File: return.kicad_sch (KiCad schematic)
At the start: 46 parts, among them IC1 LC709203F/MH, Q3 MOSFET-P, SW1 SWITCH_TACT_SMT4.6X2.8, SW2 SWITCH_TACT_SMT4.6X2.8, SW3 SW_Push, U1 ESP32-S3-MINI-1, U2 VREG_SOT23-5, U3 MCP73831/2, U4 BME280, U5 VREG_SOT23-5, X1 JSTPH, X3 USB_C

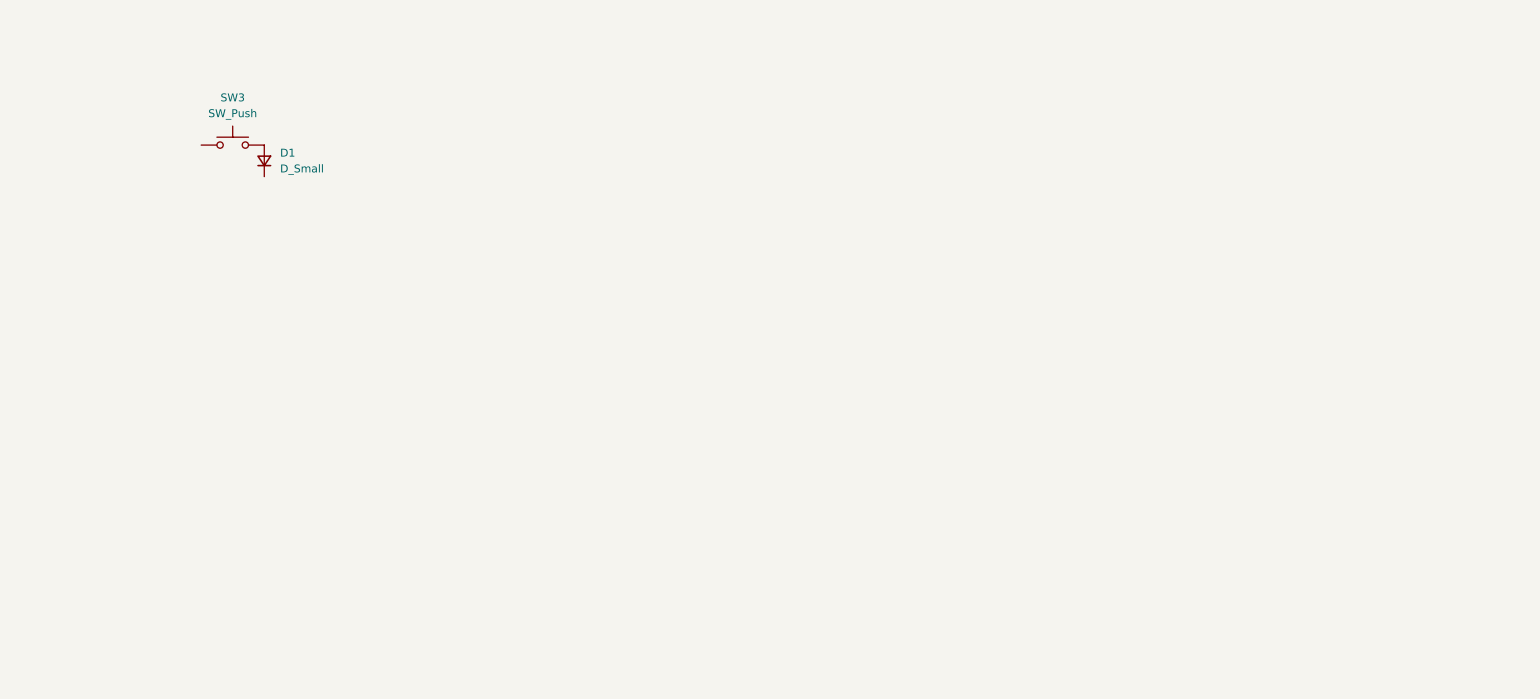
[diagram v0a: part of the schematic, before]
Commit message: Revise Schematic
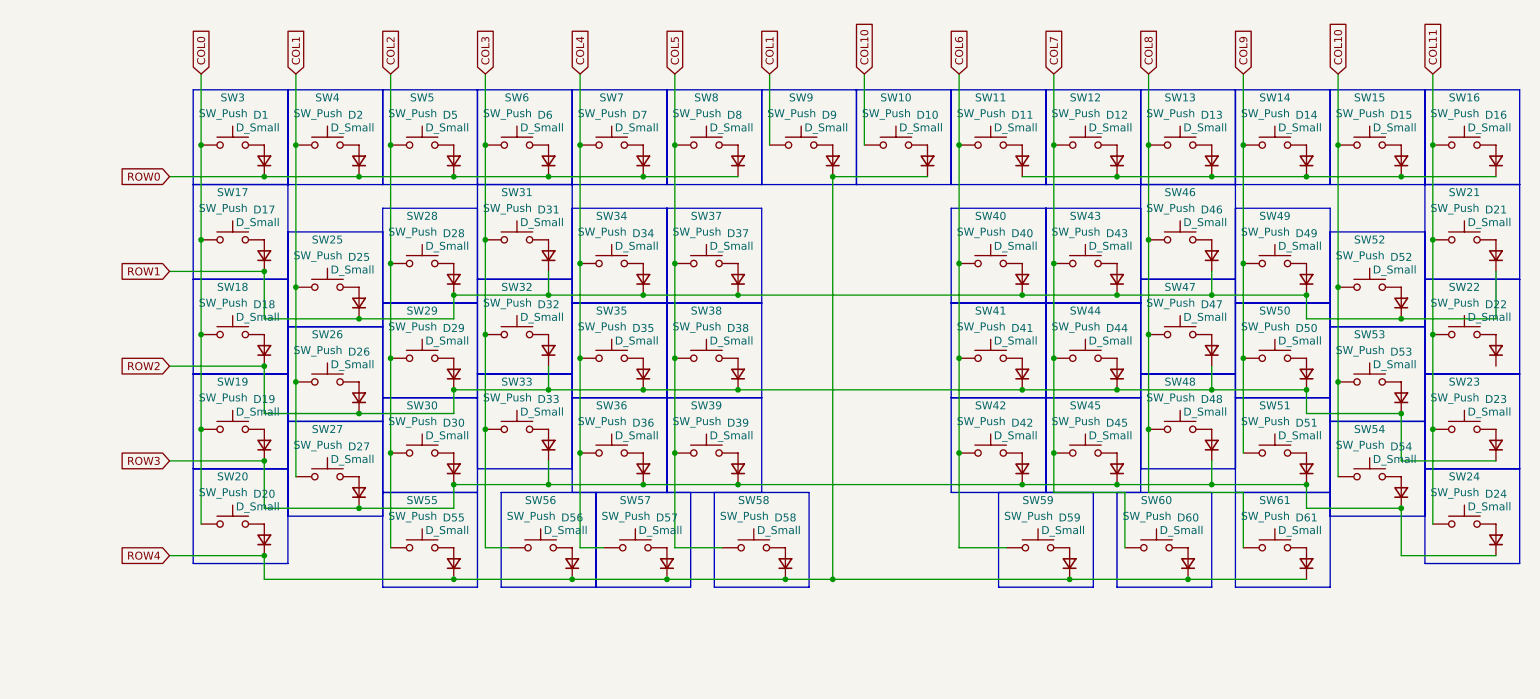
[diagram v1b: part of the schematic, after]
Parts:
- added D10, D11, D12, D13, D14, D15, D16, D17, D18, D19, D2, D20, D21, D22, D23, D24, D25, D26, D27, D28, D29, D30, D31, D32, D33, D34, D35, D36, D37, D38, D39, D40, D41, D42, D43, D44, D45, D46, D47, D48, D49, D5, D50, D51, D52, D53, D54, D55, D56, D57, D58, D59, D6, D60, D61, D7, D8, D9: D_Small, symbol Device:D_Small
- added SW10, SW11, SW12, SW13, SW14, SW15, SW16, SW17, SW18, SW19, SW20, SW21, SW22, SW23, SW24, SW25, SW26, SW27, SW28, SW29, SW30, SW31, SW32, SW33, SW34, SW35, SW36, SW37, SW38, SW39, SW4, SW40, SW41, SW42, SW43, SW44, SW45, SW46, SW47, SW48, SW49, SW5, SW50, SW51, SW52, SW53, SW54, SW55, SW56, SW57, SW58, SW59, SW6, SW60, SW61, SW7, SW8, SW9: SW_Push, symbol Switch:SW_Push
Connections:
- net ROW0: now reaches D1.1 (K)
- net ROW0: now also D2.1 (K), D5.1 (K), D6.1 (K), D7.1 (K), D8.1 (K)
- net COL0: now reaches SW3.1
- net COL0: now also SW17.1, SW18.1, SW19.1, SW20.1
- new net: D33.2 (A), SW33.2
- new net: D58.2 (A), SW58.2
- new net: D39.2 (A), SW39.2
- new net: D48.2 (A), SW48.2
- new net: D60.2 (A), SW60.2
- new net: D10.2 (A), SW10.2
- new net: D11.1 (K), D12.1 (K), D13.1 (K), D14.1 (K), D15.1 (K), D16.1 (K)
- new net: D14.2 (A), SW14.2
- new net: D20.2 (A), SW20.2
- new net: D8.2 (A), SW8.2
- new net: D11.2 (A), SW11.2
- new net: D53.2 (A), SW53.2
- new net: D28.2 (A), SW28.2
- new net: D50.2 (A), SW50.2
- new net: D38.2 (A), SW38.2
- new net: D47.2 (A), SW47.2
- new net: D9.2 (A), SW9.2
- new net: D35.2 (A), SW35.2
- new net: D41.2 (A), SW41.2
- new net: D45.2 (A), SW45.2
- new net: D22.2 (A), SW22.2
- new net: D24.2 (A), SW24.2
- new net: D61.2 (A), SW61.2
- new net: D5.2 (A), SW5.2
- new net: D44.2 (A), SW44.2
- new net: D55.2 (A), SW55.2
- new net: D19.2 (A), SW19.2
- new net: D12.2 (A), SW12.2
- new net: D6.2 (A), SW6.2
- new net: D37.2 (A), SW37.2
- new net: D27.2 (A), SW27.2
- new net: D52.2 (A), SW52.2
- new net: D29.2 (A), SW29.2
- new net: D31.2 (A), SW31.2
- new net: D21.2 (A), SW21.2
- new net: D15.2 (A), SW15.2
- new net: D46.2 (A), SW46.2
- new net: D30.2 (A), SW30.2
- new net: D26.2 (A), SW26.2
- new net: D59.2 (A), SW59.2
- new net: D43.2 (A), SW43.2
- new net: D18.2 (A), SW18.2
- new net: D23.2 (A), SW23.2
- new net: D7.2 (A), SW7.2
- new net: D56.2 (A), SW56.2
- new net: D40.2 (A), SW40.2
- new net: D17.2 (A), SW17.2
- new net: D13.2 (A), SW13.2
- new net: D42.2 (A), SW42.2
- new net: D57.2 (A), SW57.2
- new net: D51.2 (A), SW51.2
- new net: D32.2 (A), SW32.2
- new net: D36.2 (A), SW36.2
- new net: D34.2 (A), SW34.2
- new net: D25.2 (A), SW25.2
- new net: D2.2 (A), SW4.2
- new net: D54.2 (A), SW54.2
- new net: D16.2 (A), SW16.2
- new net: D49.2 (A), SW49.2
- new net COL1: SW25.1, SW26.1, SW27.1, SW4.1, SW9.1
- new net COL10: SW10.1, SW15.1, SW52.1, SW53.1, SW54.1
- new net COL11: SW16.1, SW21.1, SW22.1, SW23.1, SW24.1
- new net COL2: SW28.1, SW29.1, SW30.1, SW5.1, SW55.1
- new net COL3: SW31.1, SW32.1, SW33.1, SW56.1, SW6.1
- new net COL4: SW34.1, SW35.1, SW36.1, SW57.1, SW7.1
- new net COL5: SW37.1, SW38.1, SW39.1, SW58.1, SW8.1
- new net COL6: SW11.1, SW40.1, SW41.1, SW42.1, SW59.1
- new net COL7: SW12.1, SW43.1, SW44.1, SW45.1, SW60.1
- new net COL8: SW13.1, SW46.1, SW47.1, SW48.1, SW61.1
- new net COL9: SW14.1, SW49.1, SW50.1, SW51.1
- new net ROW1: D17.1 (K), D21.1 (K), D25.1 (K), D28.1 (K), D31.1 (K), D34.1 (K), D37.1 (K), D40.1 (K), D43.1 (K), D46.1 (K), D49.1 (K), D52.1 (K)
- new net ROW2: D18.1 (K), D23.1 (K), D26.1 (K), D29.1 (K), D32.1 (K), D35.1 (K), D38.1 (K), D41.1 (K), D44.1 (K), D47.1 (K), D50.1 (K), D53.1 (K)
- new net ROW3: D19.1 (K), D24.1 (K), D27.1 (K), D30.1 (K), D33.1 (K), D36.1 (K), D39.1 (K), D42.1 (K), D45.1 (K), D48.1 (K), D51.1 (K), D54.1 (K)
- new net ROW4: D10.1 (K), D20.1 (K), D55.1 (K), D56.1 (K), D57.1 (K), D58.1 (K), D59.1 (K), D60.1 (K), D61.1 (K), D9.1 (K)
